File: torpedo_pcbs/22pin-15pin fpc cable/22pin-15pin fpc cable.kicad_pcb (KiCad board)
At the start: 2 copper layers, 19.8 x 16 mm, 2 parts, among them J1 Conn_01x22, J2 Conn_01x15

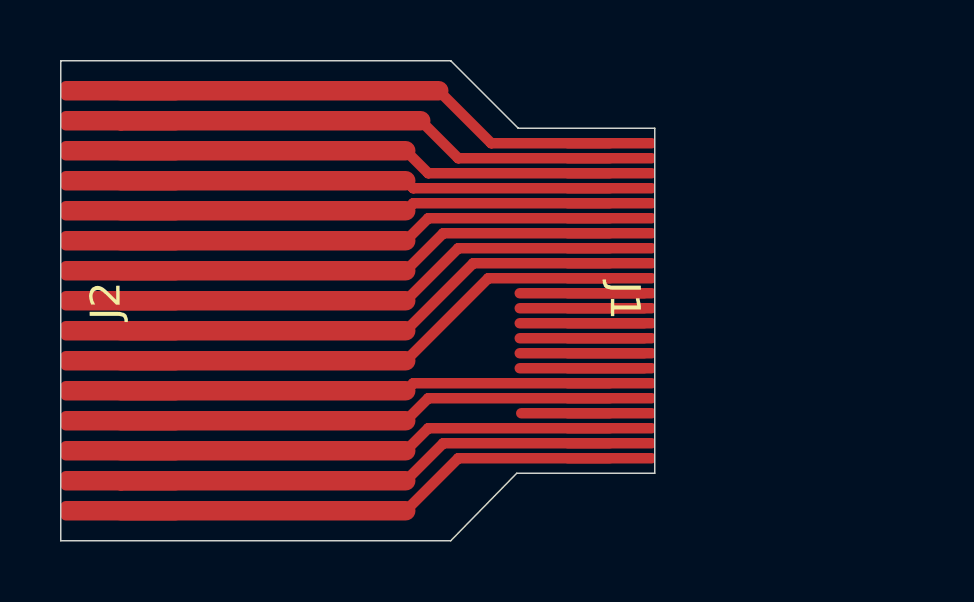
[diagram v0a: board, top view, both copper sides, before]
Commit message: June-1-2025 jlcpcb order
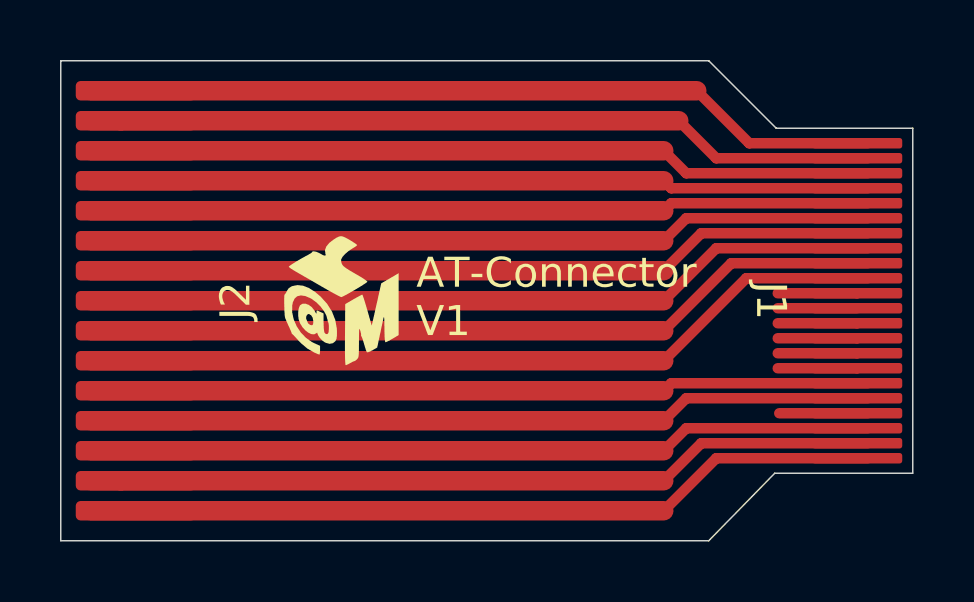
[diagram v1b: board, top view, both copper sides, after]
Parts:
- added G***: LOGO, LOGO, F.Cu at (123.2, 100.0)
- moved J1 8.25 mm to (140.4, 100.0)
- moved J2 0.50 mm to (116.4, 100.0)
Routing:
- net Net-(J1-Pin_9): track 17.2 -> 26.8 mm
- net Net-(J1-Pin_8): track 17.0 -> 26.6 mm
- net Net-(J1-Pin_7): track 16.8 -> 26.4 mm
- net Net-(J1-Pin_6): track 16.6 -> 26.2 mm
- net Net-(J1-Pin_5): track 16.4 -> 26.0 mm
- net Net-(J1-Pin_22): track 17.0 -> 26.6 mm
- net Net-(J1-Pin_21): track 16.8 -> 26.4 mm
- net Net-(J1-Pin_20): track 16.6 -> 26.2 mm
- net Net-(J1-Pin_18): track 16.6 -> 26.2 mm
- net Net-(J1-Pin_17): track 16.4 -> 26.0 mm
- net Net-(J1-Pin_10): track 17.4 -> 27.0 mm
- net Net-(J1-Pin_1): track 17.0 -> 26.6 mm
- net Net-(J1-Pin_4): track 16.4 -> 26.0 mm
- net Net-(J1-Pin_3): track 16.6 -> 26.2 mm
- net Net-(J1-Pin_2): track 16.8 -> 26.4 mm
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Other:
- board size 19.8 x 16 mm -> 28.4 x 16 mm
- board text added: "AT-Connector V1"
